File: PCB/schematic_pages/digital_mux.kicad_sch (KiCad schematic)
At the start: 9 parts

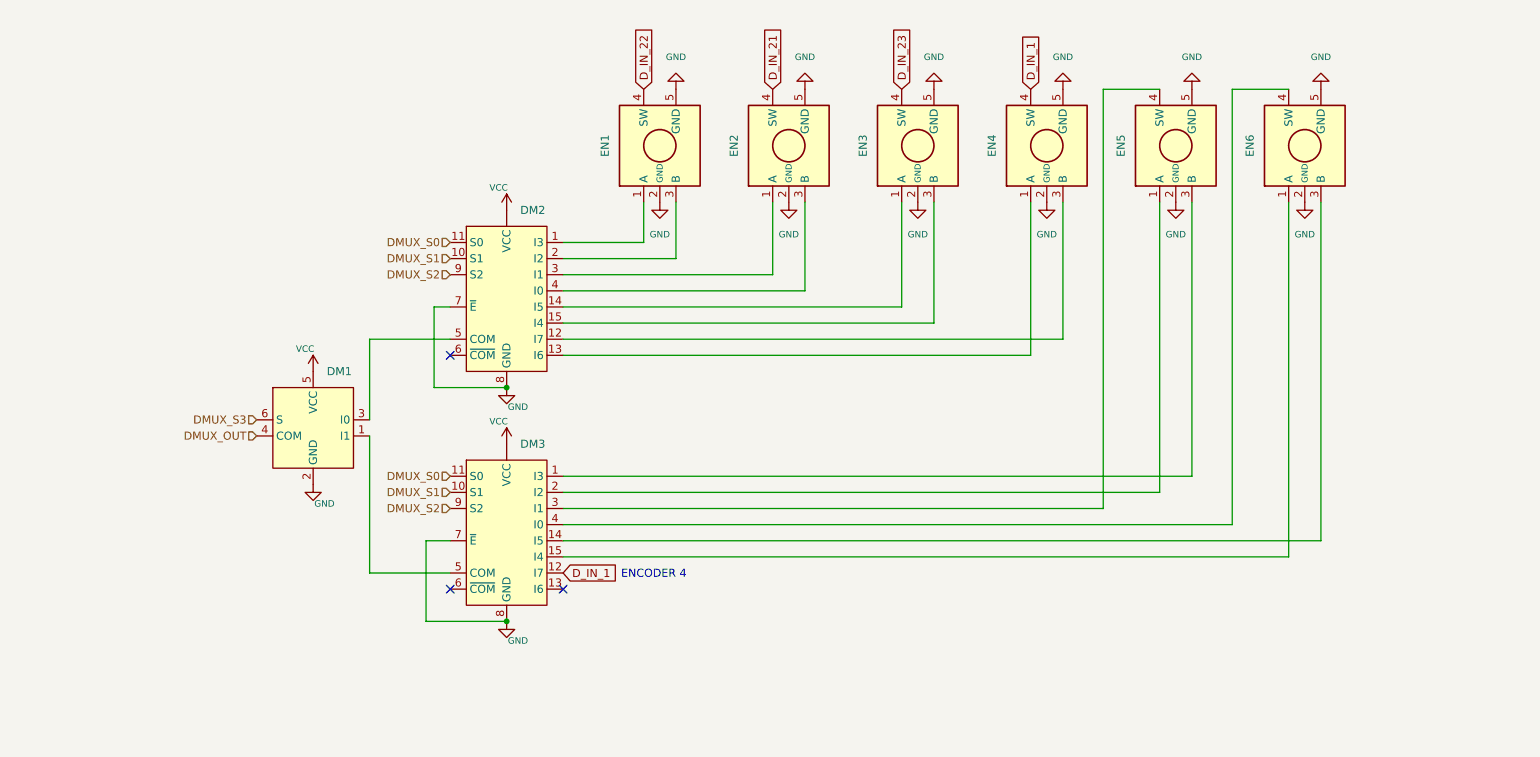
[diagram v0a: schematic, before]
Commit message: finished reworking pcb
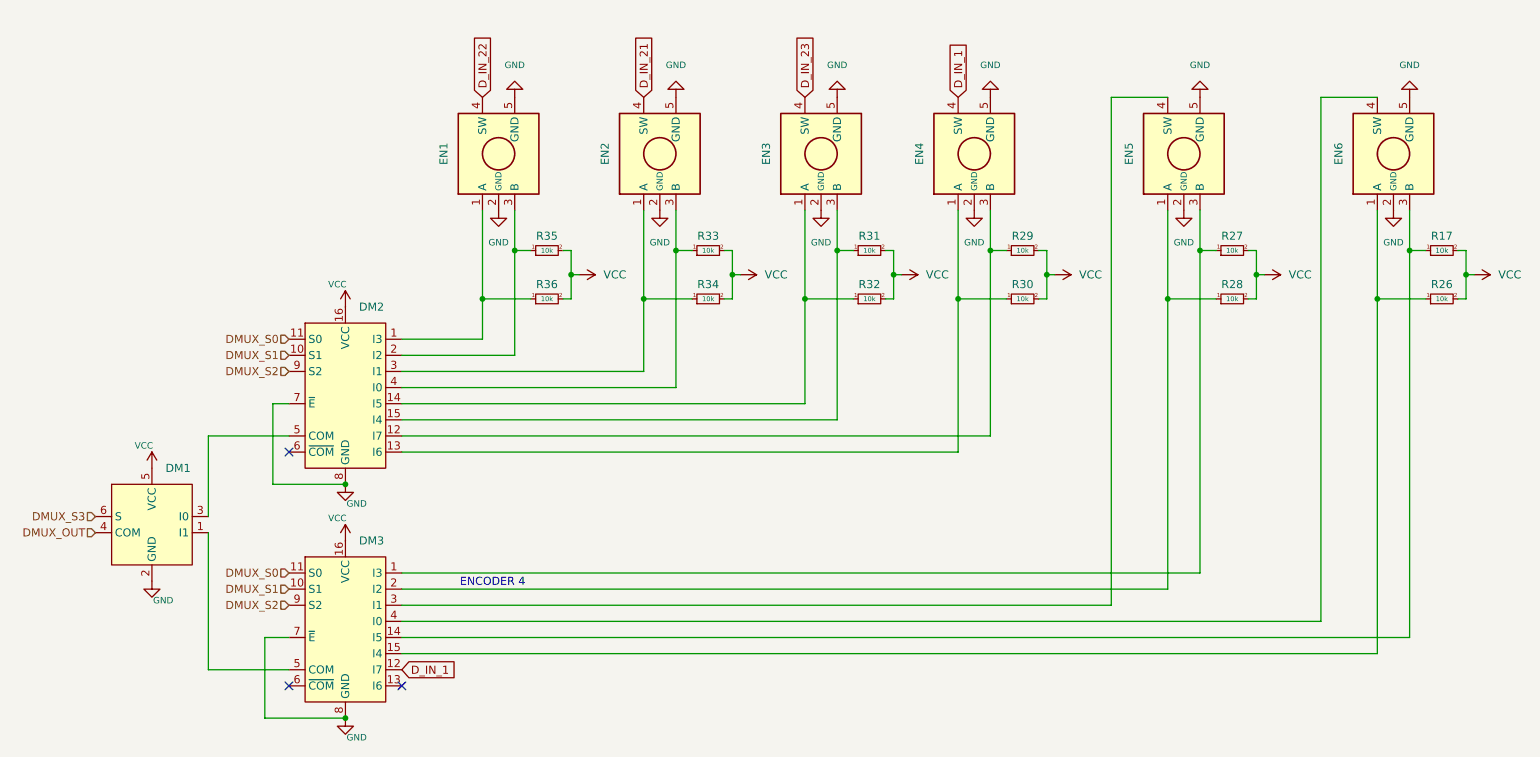
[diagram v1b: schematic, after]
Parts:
- added R17, R26, R27, R28, R29, R30, R31, R32, R33, R34, R35, R36: 10k, Footprints:0603_R, symbol Symbols:Resistor 0603
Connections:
- net VCC: now also DM2.16 (VCC), DM3.16 (VCC), R17.2, R26.2, R27.2, R28.2, R29.2, R30.2, R31.2, R32.2, R33.2, R34.2, R35.2, R36.2; no longer DM2. (VCC), DM3. (VCC)
- net at DM3.2 (I2), EN5.1 (A): now also R28.1
- net at DM3.1 (I3), EN5.3 (B): now also R27.1
- net at DM2.3 (I1), EN2.1 (A): now also R34.1
- net at DM2.4 (I0), EN2.3 (B): now also R33.1
- net at DM2.1 (I3), EN1.1 (A): now also R36.1
- net at DM2.12 (I7), EN4.3 (B): now also R29.1
- net at DM2.13 (I6), EN4.1 (A): now also R30.1
- net at DM2.14 (I5), EN3.1 (A): now also R32.1
- net at DM2.15 (I4), EN3.3 (B): now also R31.1
- net at DM2.2 (I2), EN1.3 (B): now also R35.1
- net at DM3.15 (I4), EN6.1 (A): now also R26.1
- net at DM3.14 (I5), EN6.3 (B): now also R17.1
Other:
- moved on the sheet: DM1, EN1, EN2, EN3, EN4, EN5, EN6
